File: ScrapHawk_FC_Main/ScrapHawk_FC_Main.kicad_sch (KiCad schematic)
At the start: 22 parts, among them IC1 MP1584EN-LF-Z, J1 USB_C_Receptacle_USB2.0_16P, U1 RP2040, U2 W25Q128JVS, Y1 Crystal_GND24

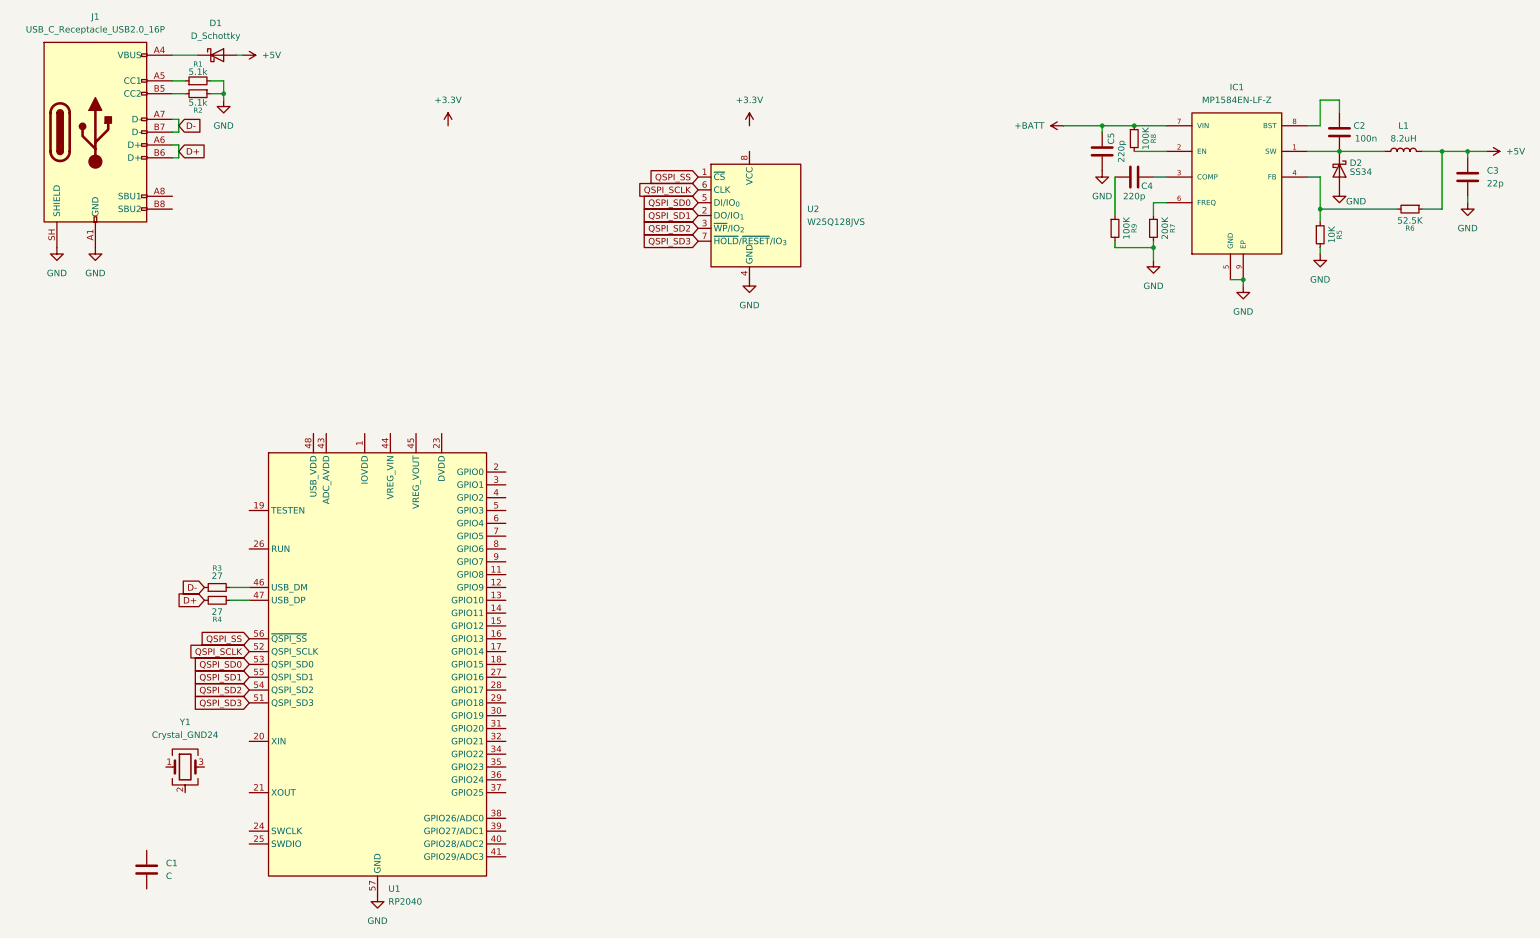
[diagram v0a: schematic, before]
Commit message: update gyro
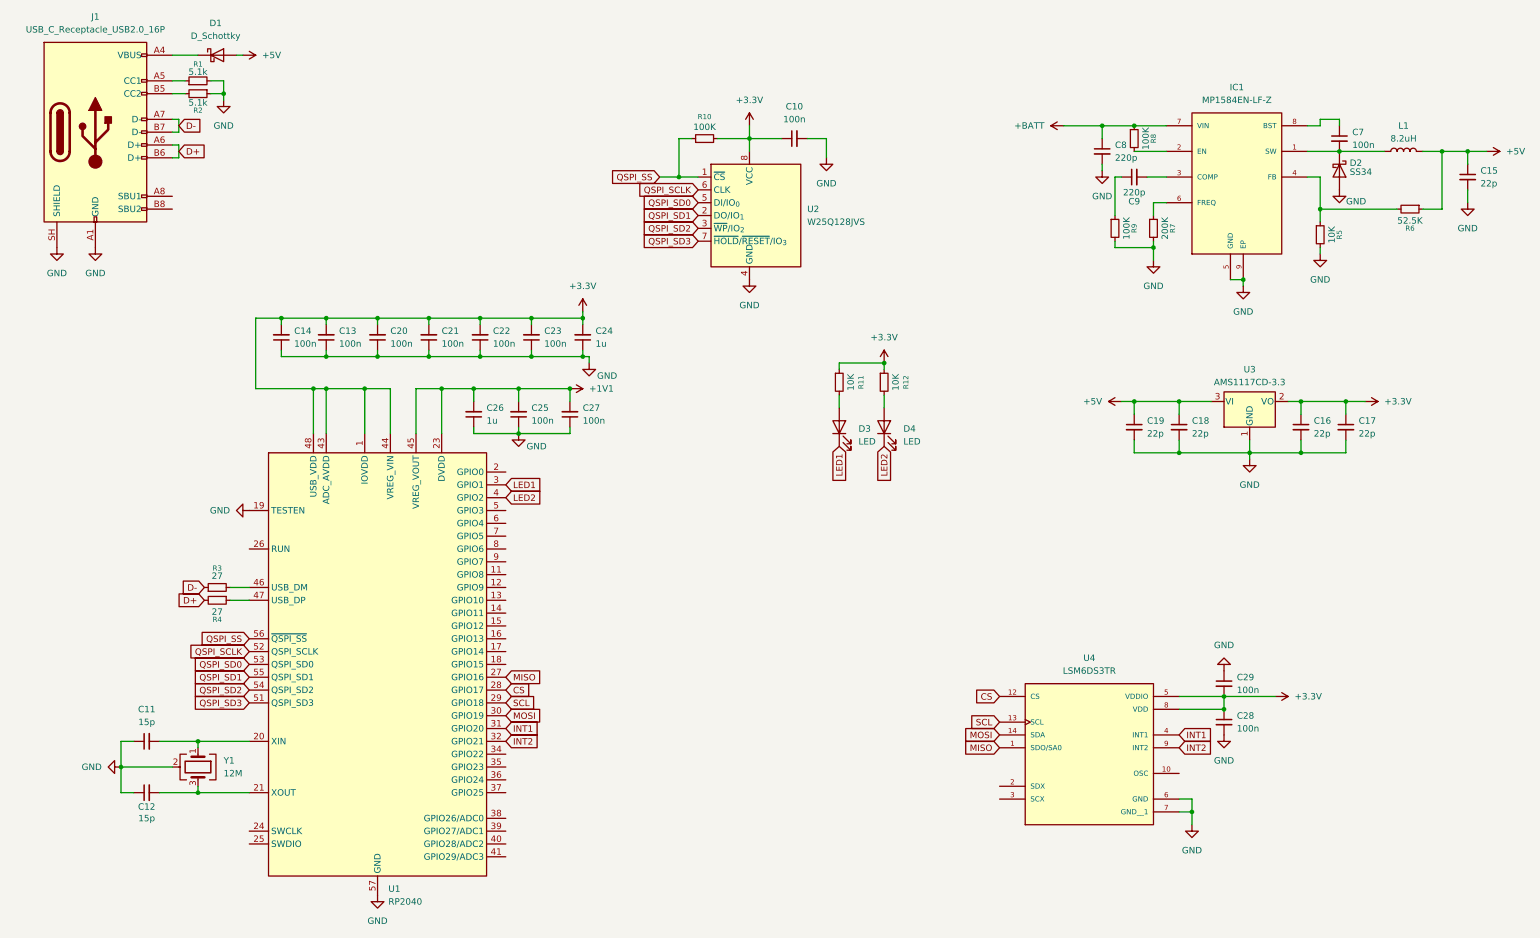
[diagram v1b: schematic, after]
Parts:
- removed C1: C, symbol Device:C
- removed C2: 100n, symbol Device:C
- removed C3: 22p, symbol Device:C
- removed C4, C5: 220p, symbol Device:C
- added C10, C13, C14, C20, C21, C22, C23, C25, C27, C28, C29, C7: 100n, Capacitor_SMD:C_0603_1608Metric, symbol Device:C_Small
- added C11, C12: 15p, Capacitor_SMD:C_0603_1608Metric, symbol Device:C_Small
- added C15, C16, C17, C18, C19: 22p, Capacitor_SMD:C_0603_1608Metric, symbol Device:C_Small
- added C24, C26: 1u, Capacitor_SMD:C_0603_1608Metric, symbol Device:C_Small
- added C8, C9: 220p, Capacitor_SMD:C_0603_1608Metric, symbol Device:C_Small
- added D3, D4: LED, Capacitor_SMD:C_0603_1608Metric, symbol Device:LED
- added R10: 100K, Resistor_SMD:R_0603_1608Metric, symbol Device:R_Small
- added R11, R12: 10K, Resistor_SMD:R_0603_1608Metric, symbol Device:R_Small
- added U3: AMS1117CD-3.3, Package_TO_SOT_SMD:SOT-223, symbol Regulator_Linear:AMS1117CD-3.3
- added U4: LSM6DS3TR, LSM6DS3TR:PQFN50P300X250X86-14N, symbol LSM6DS3TR:LSM6DS3TR
- D1: footprint (none) -> Diode_SMD:D_0805_2012Metric
- D2: footprint (none) -> Diode_SMD:D_SMC
- J1: footprint (none) -> Connector_USB:USB_C_Receptacle_G-Switch_GT-USB-7010ASV
- L1: footprint (none) -> Inductor_SMD:L_Chilisin_BMRA00050520
- R1, R2, R3, R4, R5, R6, R7, R8, R9: footprint (none) -> Resistor_SMD:R_0603_1608Metric
- Y1: value Crystal_GND24 -> 12M; footprint (none) -> Crystal:Crystal_SMD_SeikoEpson_TSX3225-4Pin_3.2x2.5mm
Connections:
- net +3.3V: now also U1.1 (IOVDD), U1.10 (IOVDD), U1.22 (IOVDD), U1.33 (IOVDD), U1.42 (IOVDD), U1.43 (ADC_AVDD), U1.44 (VREG_VIN), U1.48 (USB_VDD), U1.49 (IOVDD), U2.8 (VCC), C10.1, C13.2, C14.2, C16.1, C17.1, C20.2, C21.2, C22.2, C23.2, C24.2, C28.1, C29.2, R10.2, R11.1, R12.1, U3.2 (VO), U4.5 (VDDIO), U4.8 (VDD)
- net +5V: now also C15.1, C18.1, C19.1, U3.3 (VI)
- net +BATT: now also C8.1
- net GND: now also U1.19 (TESTEN), Y1.2 (G), Y1.4 (G), C10.2, C11.1, C12.1, C13.1, C14.1, C15.2, C16.2, C17.2, C18.2, C19.2, C20.1, C21.1, C22.1, C23.1, C24.1, C25.1, C26.1, C27.1, C28.2, C29.1, C8.2, U3.1 (GND), U4.6 (GND), U4.7 (GND__1)
- net QSPI_SS: now also R10.1
- net at R9.1: now also C9.1
- net at D2.1 (K), IC1.1 (SW), L1.1: now also C7.2
- net at IC1.3 (COMP): now also C9.2
- net at IC1.8 (BST): now also C7.1
- net at U1.20 (XIN): now also Y1.1, C11.2
- net at U1.21 (XOUT): now also Y1.3, C12.2
- net +1V1: now reaches U1.23 (DVDD), U1.50 (DVDD)
- net +1V1: now also U1.45 (VREG_VOUT), C25.2, C26.2, C27.2
- net MISO: now reaches U1.27 (GPIO16)
- net MISO: now also U4.1 (SDO/SA0)
- net CS: now reaches U1.28 (GPIO17)
- net CS: now also U4.12 (CS)
- net SCL: now reaches U1.29 (GPIO18)
- net SCL: now also U4.13 (SCL)
- net LED1: now reaches U1.3 (GPIO1)
- net LED1: now also D3.1 (K)
- net MOSI: now reaches U1.30 (GPIO19)
- net MOSI: now also U4.14 (SDA)
- net INT1: now reaches U1.31 (GPIO20)
- net INT1: now also U4.4 (INT1)
- net INT2: now reaches U1.32 (GPIO21)
- net INT2: now also U4.9 (INT2)
- net LED2: now reaches U1.4 (GPIO2)
- net LED2: now also D4.1 (K)
- new net: D4.2 (A), R12.2
- new net: D3.2 (A), R11.2
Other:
- moved on the sheet: Y1
